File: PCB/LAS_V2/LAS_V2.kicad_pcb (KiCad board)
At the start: 2 copper layers, 95 x 95 mm, 67 parts, among them J1 Screw_Terminal_01x04, J10 Conn_01x02_Pin, J11 Conn_01x02_Pin, J12 Conn_01x02_Pin, J13 Conn_01x02_Pin, J14 Conn_01x02_Pin, J2 Conn_01x03_Pin, J3 Conn_01x05_Socket, J4 Conn_01x22_Socket, J5 Conn_01x22_Socket, J6 Conn_01x02_Pin, J7 USB_C_Receptacle_USB2.0, J8 Conn_01x05, J9 Conn_01x02_Pin, K1 SRD-05VDC-SL-C, Q1 MMBT2222A, Q2 MMBT2222A, Q3 MMBT2222A, Q4 MMBT2222A, Q5 AO3400A, Q6 AO3400A, U1 ESP32-S3-WROOM-1, U2 AMS1117-3.3, U3 CH340C, U5 EL357N

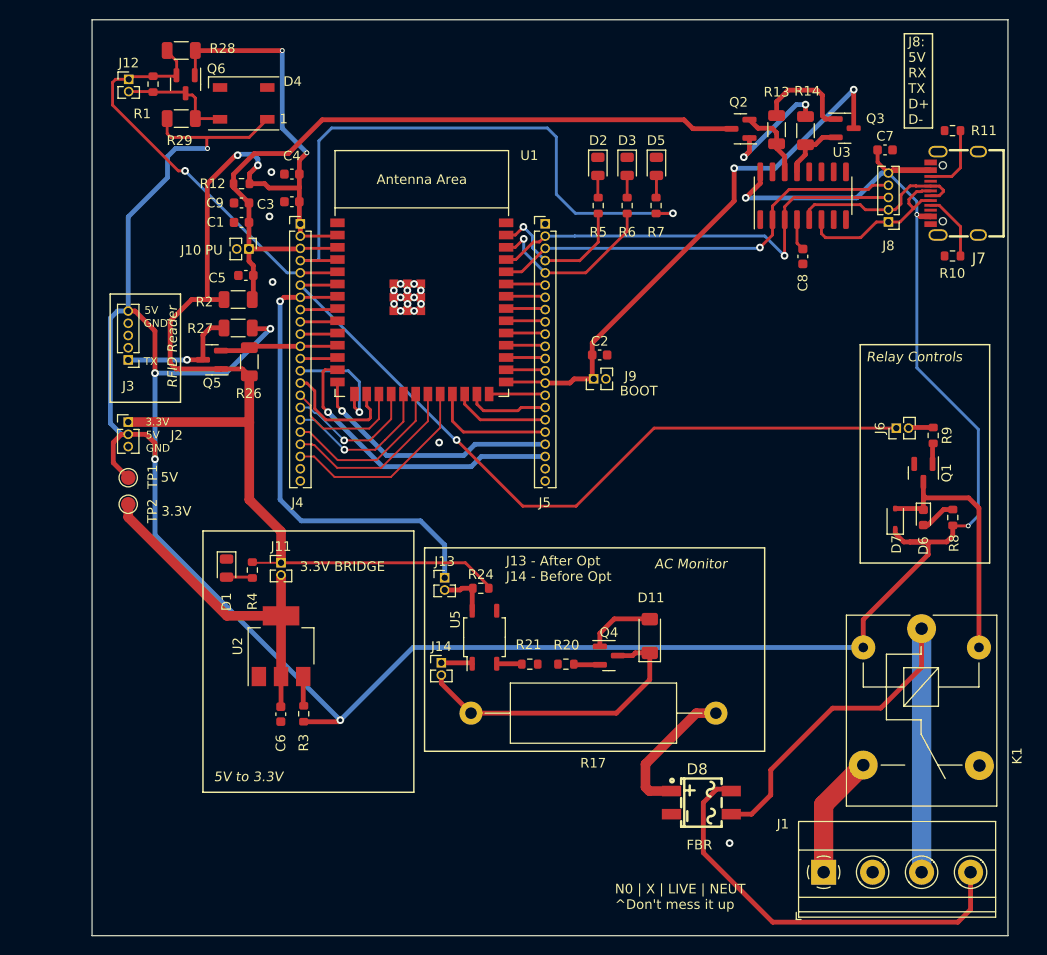
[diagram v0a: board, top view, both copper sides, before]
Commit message: Updated rme
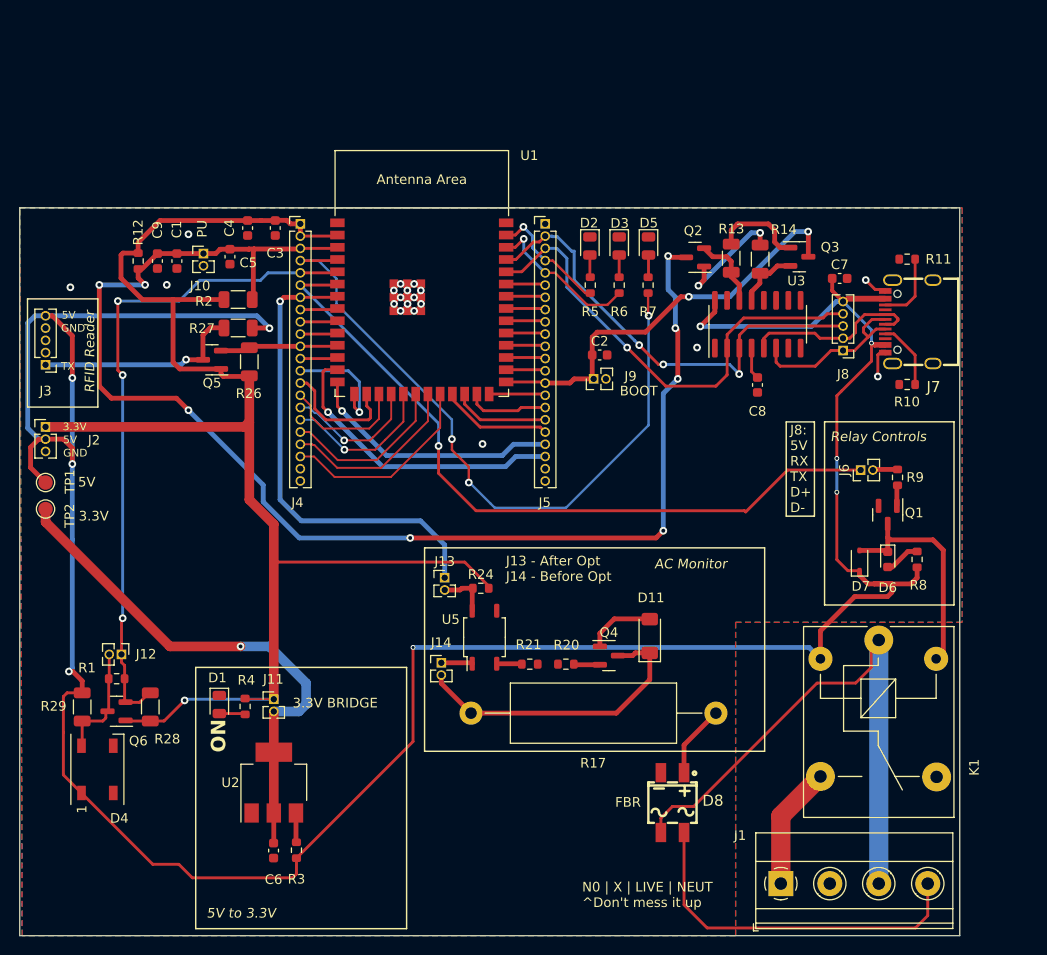
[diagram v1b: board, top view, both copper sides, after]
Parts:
- moved D4 70.7 mm to (115.5, 127.8), turned to 90 degrees
- moved R28 68.2 mm to (121.0, 121.3), turned to 90 degrees
- moved Q6 65.4 mm to (117.5, 121.7), turned to 180 degrees
- moved R29 61.9 mm to (114.0, 121.3), turned to -90 degrees
- moved R1 61.8 mm to (117.5, 118.3), turned to 0 degrees
- moved J12 59.7 mm to (118.0, 115.8), turned to -90 degrees
- moved C6 14.2 mm to (133.8, 136.2)
- moved D1 14.2 mm to (128.2, 121.0)
- moved U2 14.2 mm to (133.8, 129.1)
- moved J11 14.2 mm to (133.8, 120.5)
- moved R3 14.2 mm to (136.2, 136.1)
- moved R4 14.2 mm to (130.9, 121.2)
- moved R13 14.1 mm to (181.3, 74.7)
- moved J8 14.1 mm to (192.9, 84.3)
- moved C7 14.1 mm to (192.5, 76.8)
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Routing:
- net /CHIP_PU: track 77.5 -> 141.5 mm, vias 0 -> 8
- net /DIN_3.3: track 43.1 -> 69.3 mm, vias 1 -> 3
- net Net-(J11-Pin_2): track 35.1 -> 54.8 mm, vias 0 -> 1
- net /BOOT_SEL: track 57.1 -> 43.2 mm
- net /+3.3V: track 142.0 -> 154.3 mm, vias 4 -> 1
- net /TX_RFID: track 12.8 -> 21.6 mm
- net /GPIO4: track 64.3 -> 72.3 mm, vias 1 -> 3
- net Net-(D8-+): track 14.8 -> 7.55 mm
- net /NEUTRAL: track 43.9 -> 37.6 mm
- net GND: track 0.00 -> 6.20 mm, vias 17 -> 19
- net /RXD0: track 45.1 -> 49.2 mm
- net /GPIO1: track 15.9 -> 12.6 mm
- net Net-(D6-K): track 26.6 -> 23.8 mm
- net /GPIO2: track 18.8 -> 16.2 mm
- net /GPIO6: track 78.6 -> 76.6 mm
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- added copper zone on B.Cu, net GND
- added copper zone on F.Cu, net GND
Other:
- board size 95 x 95 mm -> 97.5 x 75.5 mm
- board text added: "ON"
